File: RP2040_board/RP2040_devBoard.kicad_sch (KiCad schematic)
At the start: 38 parts, among them J1 USB_B_Micro, J2 Conn_01x20_Male, J3 Conn_01x20_Male, J4 Conn_01x03_Male, SW1 SW_Push, U1 RP2040, U2 AMS1117, U3 W25Q128JVS, Y1 Crystal

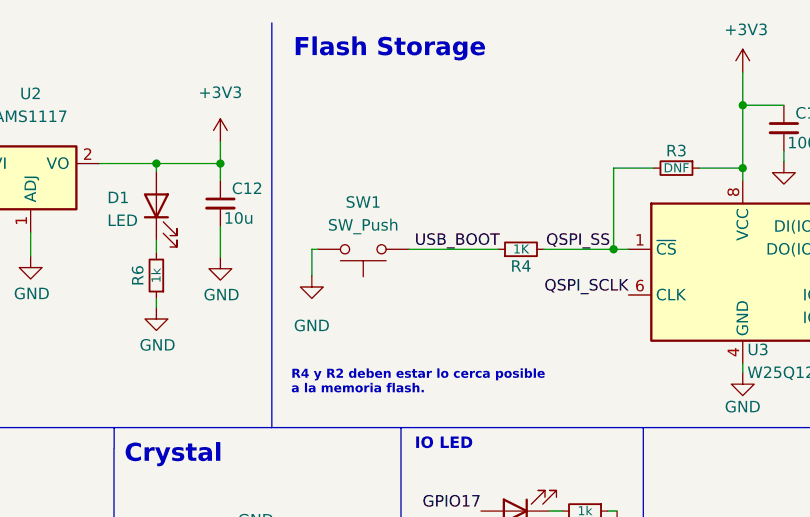
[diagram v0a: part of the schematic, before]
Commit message: board finish
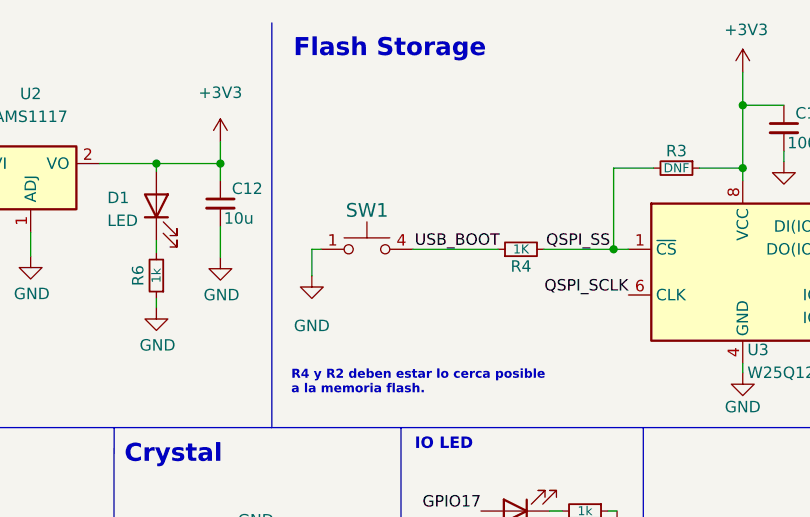
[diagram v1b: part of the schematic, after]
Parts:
- removed SW1: SW_Push, Tactile_SW:SW_PTS636_SMT-G_5_CNK, symbol Switch:SW_Push
- added SW1: PTS815_SJM_250_SMTR_LFS, FOOTPRINTS_s1:SW4_PTS815 SJM 250 SMTR LFS_CNK, symbol PTS815:PTS815_SJM_250_SMTR_LFS
- D1, D3: footprint LED_SMD:LED_1206_3216Metric -> LED_SMD:LED_0603_1608Metric
- Y1: footprint Crystal:Crystal_SMD_HC49-SD -> MCU_RaspberryPi_and_Boards:Crystal_SMD_HC49-US
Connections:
- net GND: now also SW1.1
- net USB_BOOT: now also SW1.4
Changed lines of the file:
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@@
+    (stroke (width 0) (type default) (color 0 0 0 0))
+  )
+  (wire (pts (xy 214.249 37.338) (xy 215.2904 37.338))
     (stroke (width 0) (type default) (color 0 0 0 0))
   )
@@
     (stroke (width 0) (type default) (color 0 0 0 0))
   )
-  (wire (pts (xy 214.884 37.338) (xy 214.249 37.338))
-    (stroke (width 0) (type default) (color 0 0 0 0))
-  )
   (wire (pts (xy 164.211 27.813) (xy 170.942 27.813))
     (stroke (width 0) (type default) (color 0 0 0 0))
@@
     (stroke (width 0) (type default) (color 0 0 0 0))
   )
-  (wire (pts (xy 225.044 37.338) (xy 234.95 37.338))
+  (wire (pts (xy 225.4758 37.338) (xy 234.95 37.338))
     (stroke (width 0) (type default) (color 0 0 0 0))
   )
@@
       (effects (font (size 1.27 1.27)) (justify right))
     )
-    (property "Footprint" "LED_SMD:LED_1206_3216Metric" (id 2) (at 196.977 32.512 0)
+    (property "Footprint" "LED_SMD:LED_0603_1608Metric" (id 2) (at 196.977 32.512 0)
       (effects (font (size 1.27 1.27)) hide)
     )
@@
     (property "Reference" "Y1" (id 0) (at 208.534 76.708 0))
     (property "Value" "Crystal" (id 1) (at 208.534 84.074 0))
-    (property "Footprint" "Crystal:Crystal_SMD_HC49-SD" (id 2) (at 208.534 80.391 0)
+    (property "Footprint" "MCU_RaspberryPi_and_Boards:Crystal_SMD_HC49-US" (id 2) (at 208.534 80.391 0)
       (effects (font (size 1.27 1.27)) hide)
     )
@@
     )
   )
-  (symbol (lib_id "Switch:SW_Push") (at 219.964 37.338 0) (mirror x) (unit 1)
-    (in_bom yes) (on_board yes) (fields_autoplaced)
-    (property "Reference" "SW1" (id 0) (at 219.964 32.131 0))
-    (property "Value" "SW_Push" (id 1) (at 219.964 34.671 0))
-    (property "Footprint" "Tactile_SW:SW_PTS636_SMT-G_5_CNK" (id 2) (at 219.964 42.418 0)
-      (effects (font (size 1.27 1.27)) hide)
-    )
-    (property "Datasheet" "~" (id 3) (at 219.964 42.418 0)
-      (effects (font (size 1.27 1.27)) hide)
-    )
-    (pin "1")
-    (pin "2")
-  )
   (symbol (lib_id "power:GND") (at 183.388 88.519 0) (unit 1)
     (in_bom yes) (on_board yes)
@@
     (pin "1")
     (pin "2")
+  )
+  (symbol (lib_id "PTS815:PTS815_SJM_250_SMTR_LFS") (at 181.0766 32.3596 0) (unit 1)
+    (in_bom yes) (on_board yes) (fields_autoplaced)
+    (property "Reference" "SW1" (id 0) (at 220.3831 33.02 0)
+      (effects (font (size 1.524 1.524)))
+    )
+    (property "Value" "PTS815_SJM_250_SMTR_LFS" (id 1) (at 220.3831 32.2326 0)
+      (effects (font (size 1.524 1.524)) hide)
+    )
+    (property "Footprint" "FOOTPRINTS_s1:SW4_PTS815 SJM 250 SMTR LFS_CNK" (id 2) (at 219.5576 41.6052 0)
+      (effects (font (size 1.27 1.27) italic) hide)
+    )
+    (property "Datasheet" "PTS815 SJM 250 SMTR LFS" (id 3) (at 181.0766 32.3596 0)
+      (effects (font (size 1.27 1.27) italic) hide)
+    )
+    (pin "1")
+    (pin "4")
   )
   (symbol (lib_id "Connector:Conn_01x03_Male") (at 162.179 135.001 0) (unit 1)
@@
       (effects (font (size 1.27 1.27)) (justify right))
     )
-    (property "Footprint" "LED_SMD:LED_1206_3216Metric" (id 2) (at 236.855 66.421 0)
+    (property "Footprint" "LED_SMD:LED_0603_1608Metric" (id 2) (at 236.855 66.421 0)
       (effects (font (size 1.27 1.27)) hide)
     )
@@
     )
     (path "/1d380f75-9d96-4cb3-80b1-0161eae10300"
-      (reference "D1") (unit 1) (value "LED") (footprint "LED_SMD:LED_1206_3216Metric")
+      (reference "D1") (unit 1) (value "LED") (footprint "LED_SMD:LED_0603_1608Metric")
     )
     (path "/ee381a3f-e4a8-445d-97f7-36bc3fc74da6"
-      (reference "D3") (unit 1) (value "LED") (footprint "LED_SMD:LED_1206_3216Metric")
+      (reference "D3") (unit 1) (value "LED") (footprint "LED_SMD:LED_0603_1608Metric")
     )
     (path "/8305abe2-9ec2-40c5-b546-27ce019c1e90"
@@
       (reference "R8") (unit 1) (value "1k") (footprint "Resistor_SMD:R_0603_1608Metric")
     )
-    (path "/838cf614-b2e2-42f7-b700-9259c521d935"
-      (reference "SW1") (unit 1) (value "SW_Push") (footprint "Tactile_SW:SW_PTS636_SMT-G_5_CNK")
+    (path "/9e7bf311-c338-4c22-89d8-9b6c735a03ce"
+      (reference "SW1") (unit 1) (value "PTS815_SJM_250_SMTR_LFS") (footprint "FOOTPRINTS_s1:SW4_PTS815 SJM 250 SMTR LFS_CNK")
     )
     (path "/d94772be-f29e-4993-b418-3d2f2b018854"
@@
     )
     (path "/2d03d970-711c-47fd-8204-f3fce42059d8"
-      (reference "Y1") (unit 1) (value "Crystal") (footprint "Crystal:Crystal_SMD_HC49-SD")
-    )
-  )
+      (reference "Y1") (unit 1) (value "Crystal") (footprint "MCU_RaspberryPi_and_Boards:Crystal_SMD_HC49-US")
+    )
+  )
